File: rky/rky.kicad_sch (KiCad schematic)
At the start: 60 parts, among them J1 Conn_01x02_Male, J2 Li-Ion 3.7 CONN, J3 USB_C_Receptacle_USB2.0, J4 Conn_01x04_Male, J5 Conn_02x03_Odd_Even, SW1 SW_SPDT, U2 SSD1306, U3 ESP8266-12E/ESP-12E, U4 LM3940IMP-3.3/NOPB, U5 TP4056, U6 NRF24L01, Y1 16MHZ

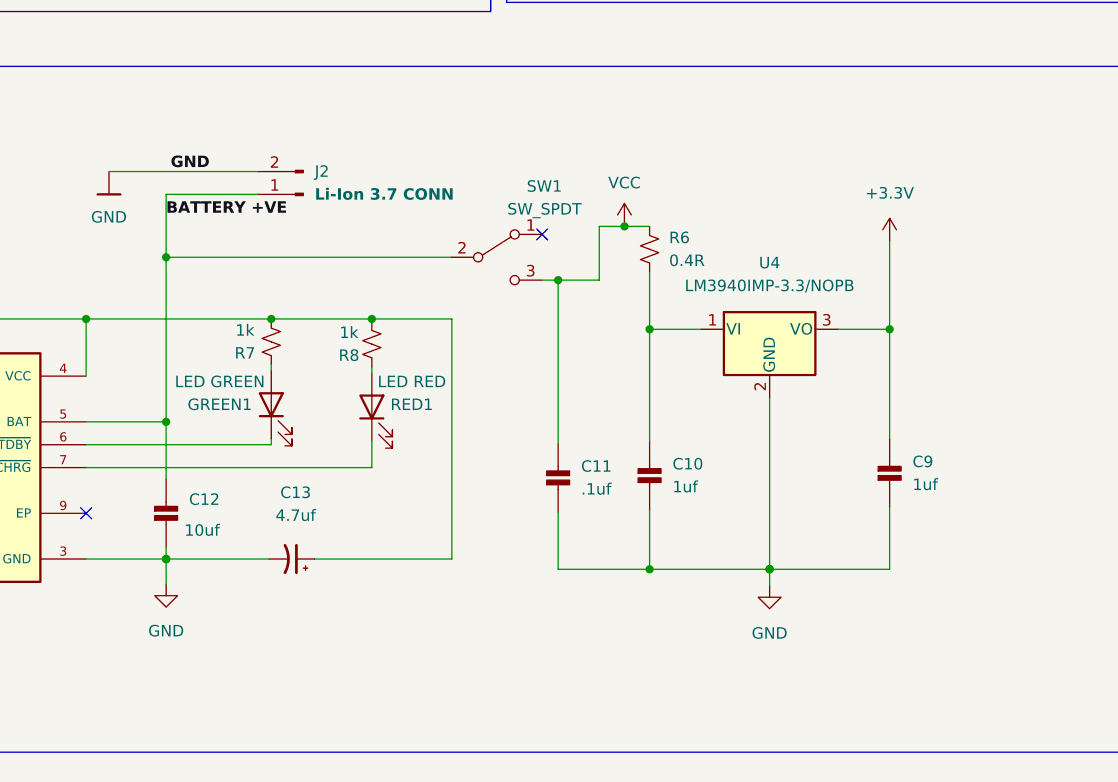
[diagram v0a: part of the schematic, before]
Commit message: add render folder
kicad 3d render image folder add
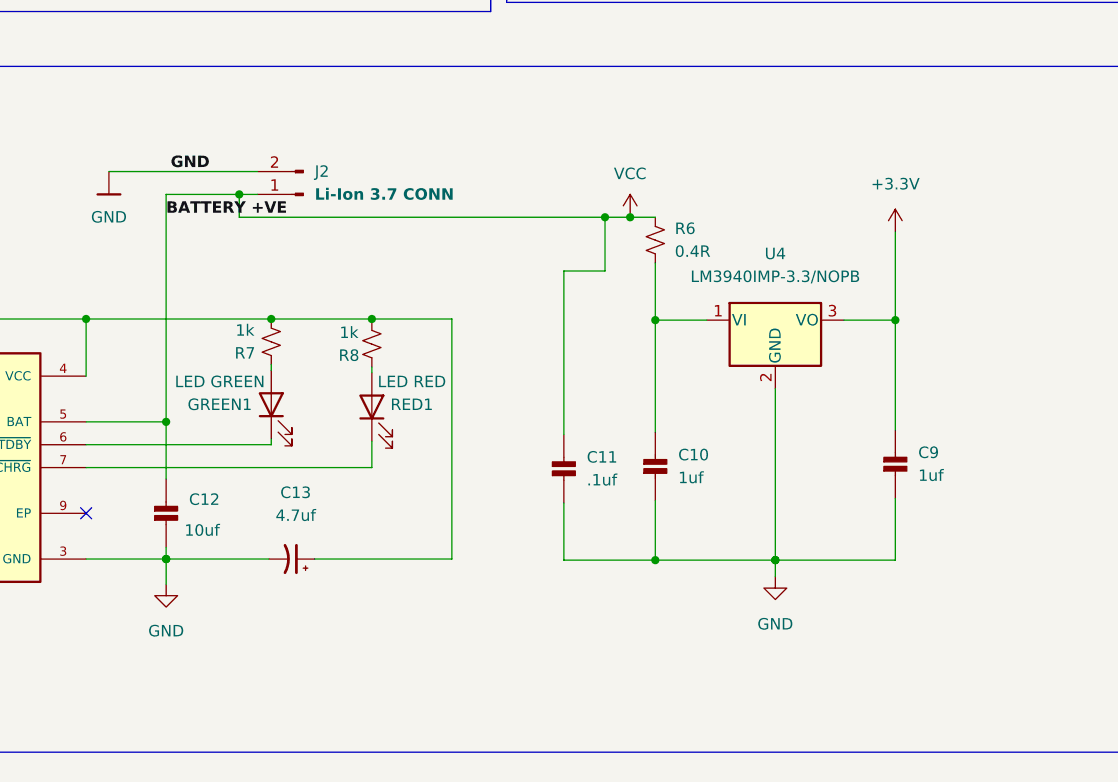
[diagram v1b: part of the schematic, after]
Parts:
- removed SW1: SW_SPDT, Button_Switch_SMD:SW_SPDT_PCM12, symbol Switch:SW_SPDT
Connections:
- net BATTERY +VE is gone; now on net VCC: C12.1 (P$1), J2.1 (Pin_1), U5.5 (BAT)
- no-connect marks 25 -> 24
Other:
- moved on the sheet: C10, C11, C9, R6, U4
